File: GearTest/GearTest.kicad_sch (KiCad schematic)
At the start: 8 parts, among them J1 Jack-DC, J2 Conn_01x02_Socket, M1 Motor_DC, M2 Motor_DC, Q1 IRLZ44N, U1 WeAct BlackPill STM32F411C_C-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, U2 INA219

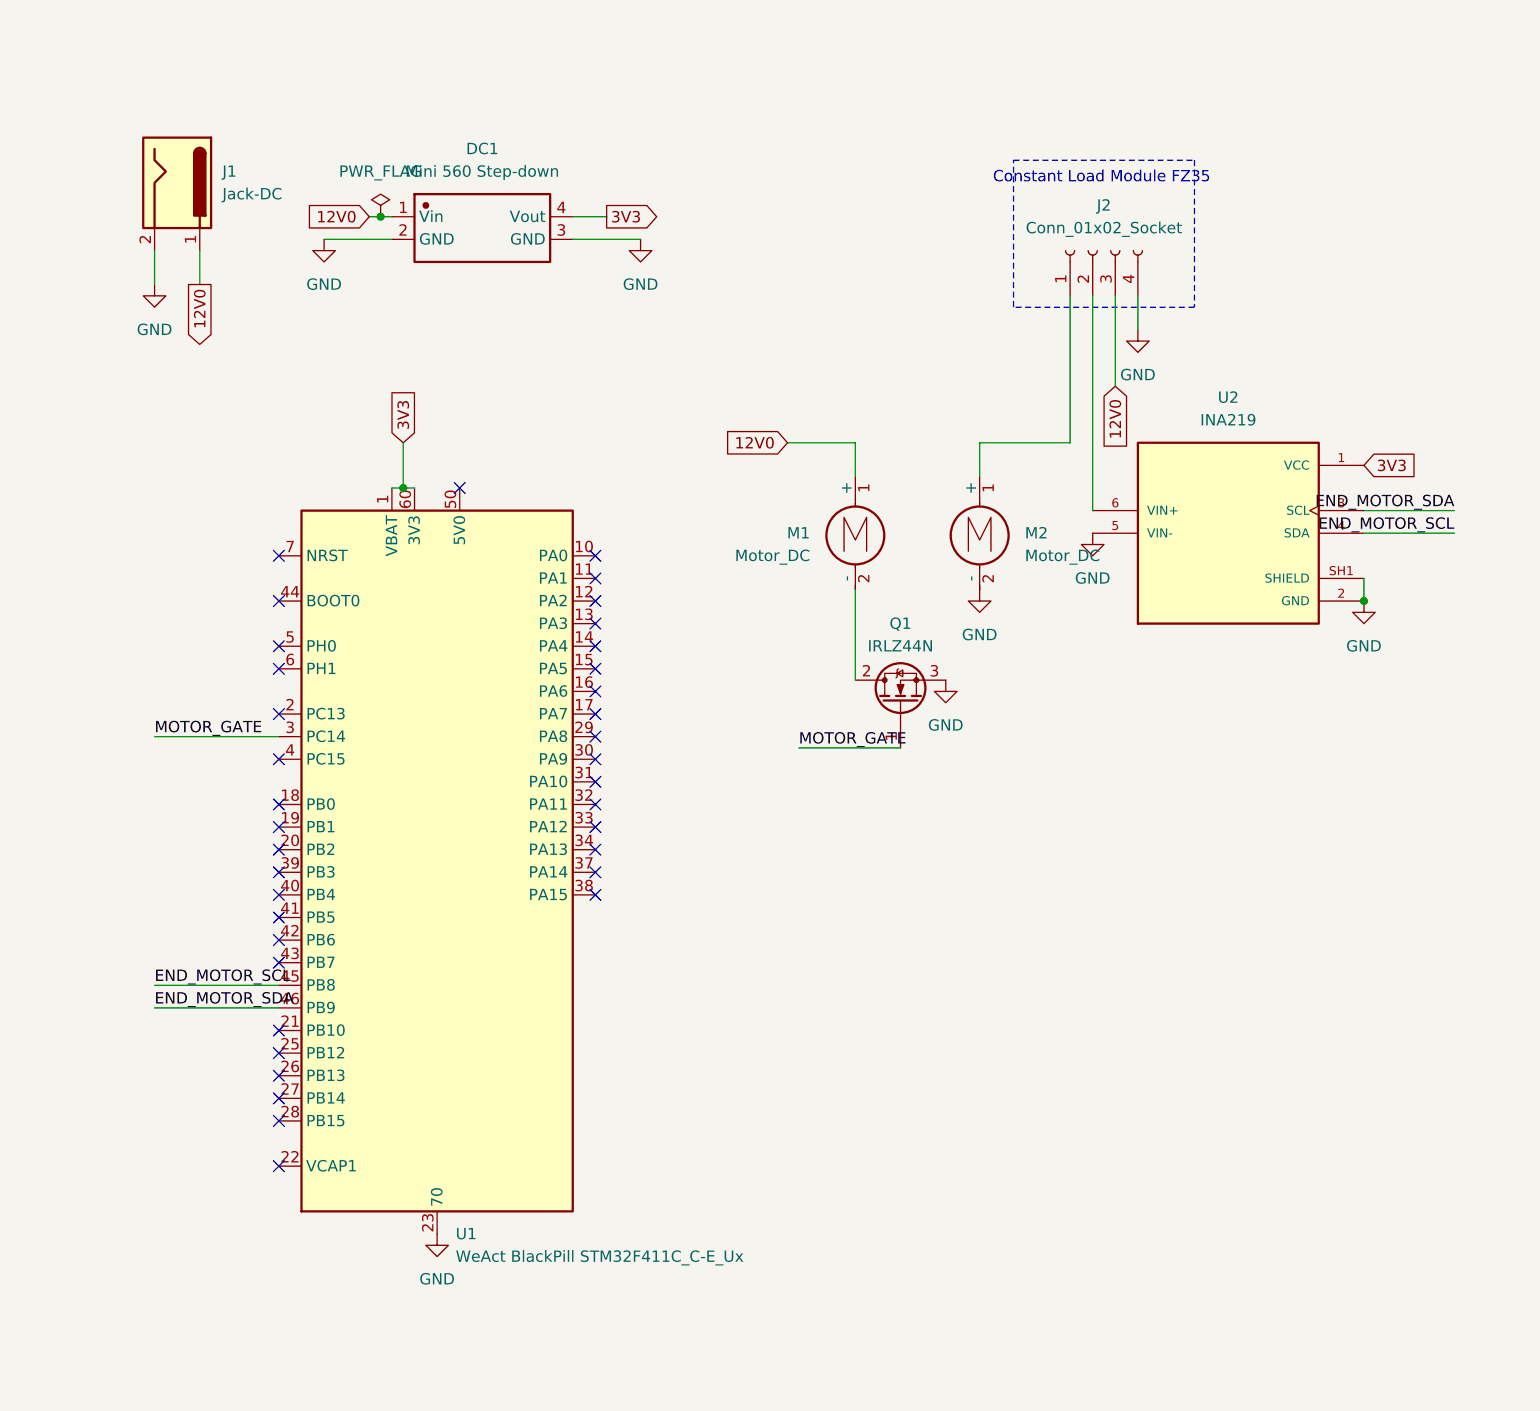
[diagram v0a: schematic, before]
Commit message: dev
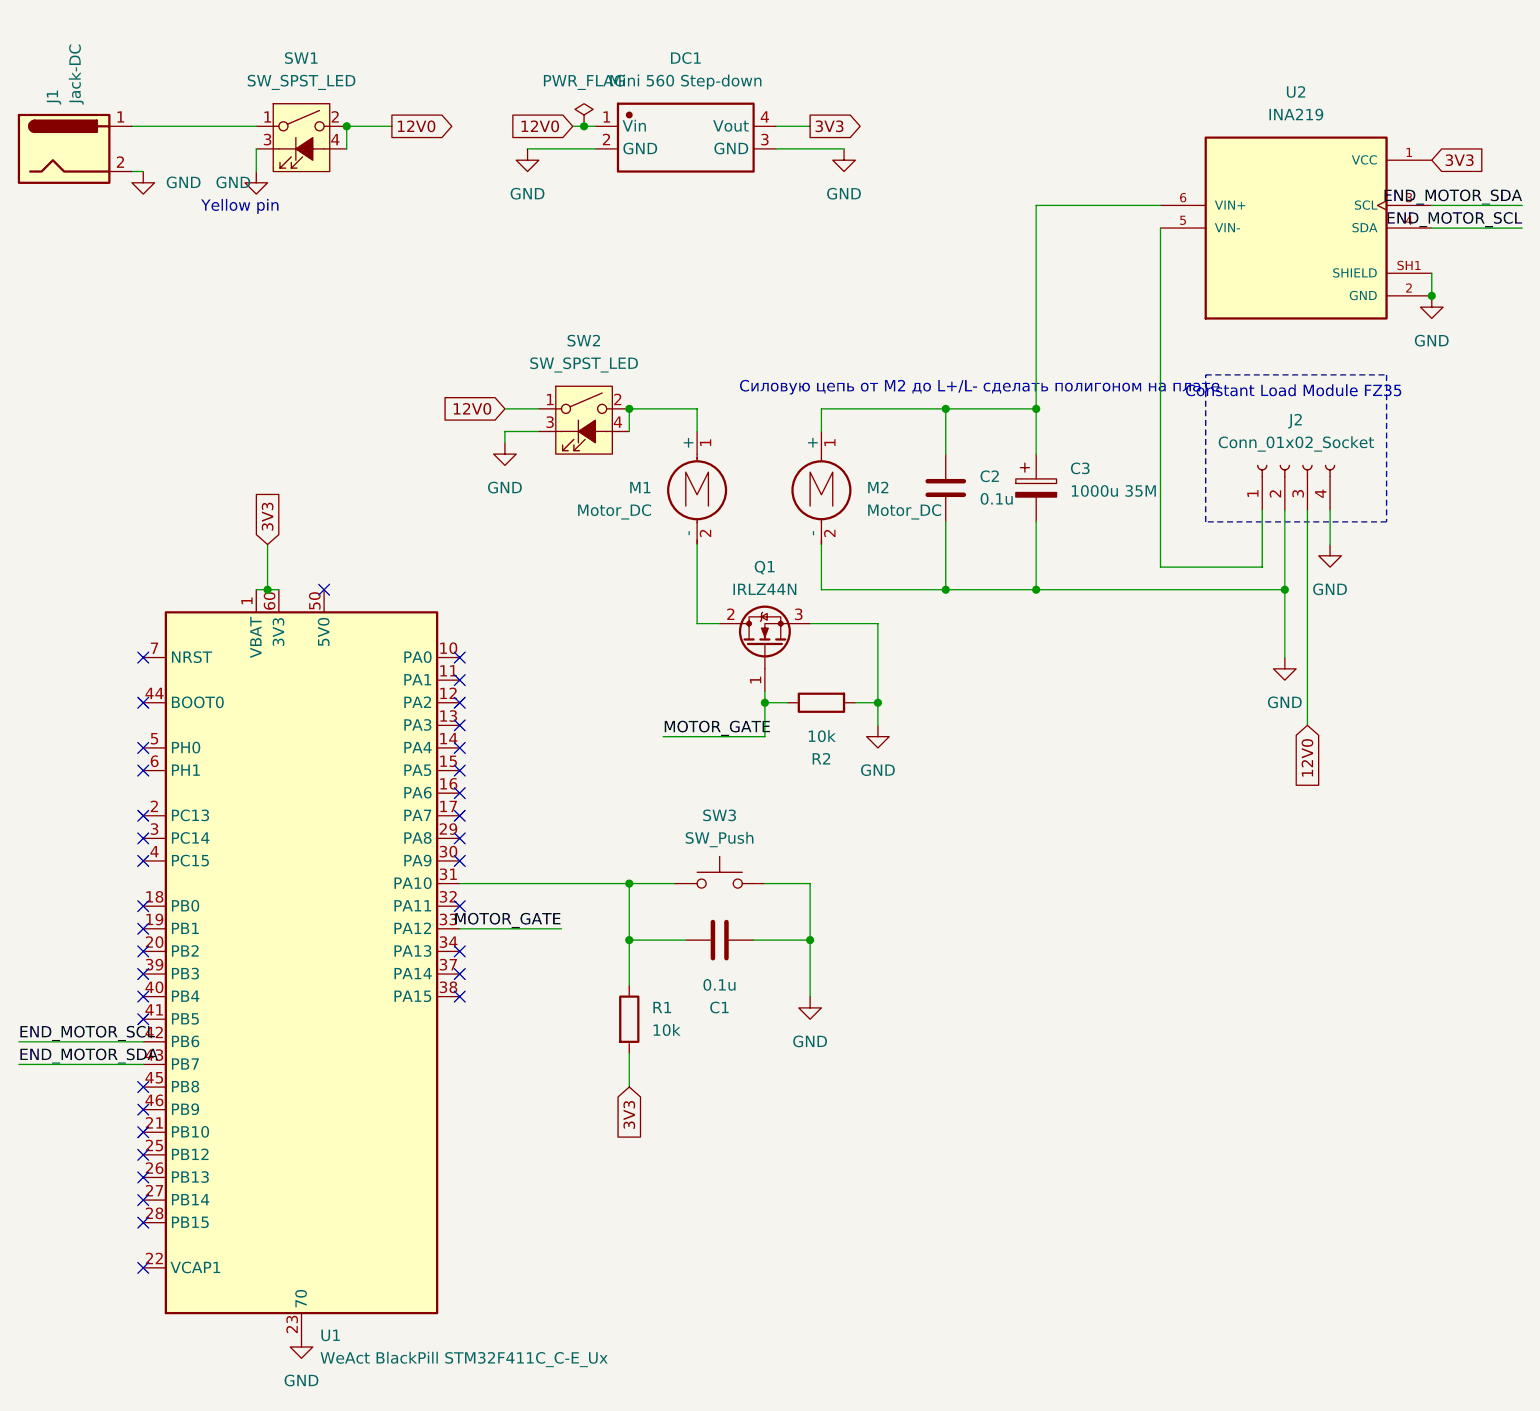
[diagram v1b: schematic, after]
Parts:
- added C1, C2: 0.1u, Capacitor_SMD:C_0805_2012Metric_Pad1.18x1.45mm_HandSolder, symbol Device:C
- added C3: 1000u 35М, Capacitor_THT:CP_Radial_D13.0mm_P5.00mm, symbol Device:C_Polarized
- added R1: 10k, Resistor_SMD:R_0603_1608Metric_Pad0.98x0.95mm_HandSolder, symbol Device:R
- added R2: 10k, symbol Device:R
- added SW1, SW2: SW_SPST_LED, TerminalBlock_Phoenix:TerminalBlock_Phoenix_MPT-0,5-3-2.54_1x03_P2.54mm_Horizontal, symbol Switch:SW_SPST_LED
- added SW3: SW_Push, TerminalBlock_Phoenix:TerminalBlock_Phoenix_MPT-0,5-2-2.54_1x02_P2.54mm_Horizontal, symbol Switch:SW_Push
- M1, M2: footprint Connector_Wire:SolderWire-0.75sqmm_1x02_P7mm_D1.25mm_OD3.5mm -> TerminalBlock_Phoenix:TerminalBlock_Phoenix_MPT-0,5-2-2.54_1x02_P2.54mm_Horizontal
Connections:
- net 12V0: now also SW1.2, SW1.4 (A), SW2.1; no longer J1.1, M1.1 (+)
- net 3V3: now also R1.2
- net END_MOTOR_SCL: now also U1.42 (PB6); no longer U1.45 (PB8)
- net END_MOTOR_SDA: now also U1.43 (PB7); no longer U1.46 (PB9)
- net GND: now also J2.2 (Pin_2), C1.2, C2.2, C3.2, R2.2, SW1.3 (K), SW2.3 (K), SW3.2; no longer U2.5 (VIN-), U2.VIN-
- net MOTOR_GATE: now also U1.33 (PA12), R2.1; no longer U1.3 (PC14)
- net at M2.1 (+): now also U2.6 (VIN+), U2.VIN+, C2.1, C3.1; no longer J2.1 (Pin_1)
- net at U1.31 (PA10): now also C1.1, R1.1, SW3.1
- new net: J1.1, SW1.1
- new net: M1.1 (+), SW2.2, SW2.4 (A)
- new net: J2.1 (Pin_1), U2.5 (VIN-), U2.VIN-
- no-connect marks 37 -> 36
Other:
- note added: "Yellow pin"
- note added: "Силовую цепь от M2 до L+/L- сделать полигоном на плате"
- moved on the sheet: DC1, J1, J2, M1, M2, Q1, U1, U2
